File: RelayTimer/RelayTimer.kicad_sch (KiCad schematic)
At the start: 20 parts, among them J1 Jack-DC, J2 Relay_Con, Q1 2N3904, U1 ATtiny85-20P

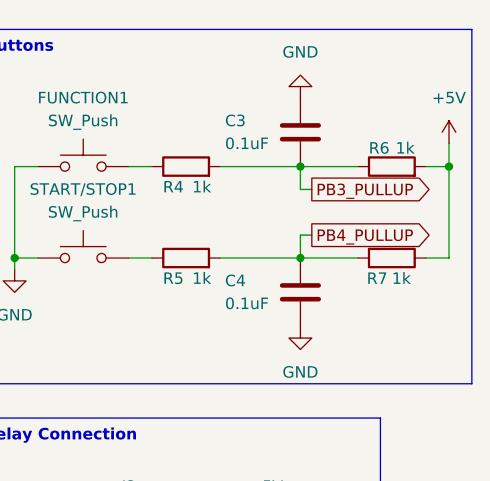
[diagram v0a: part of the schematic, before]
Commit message: minor update to KiCad project
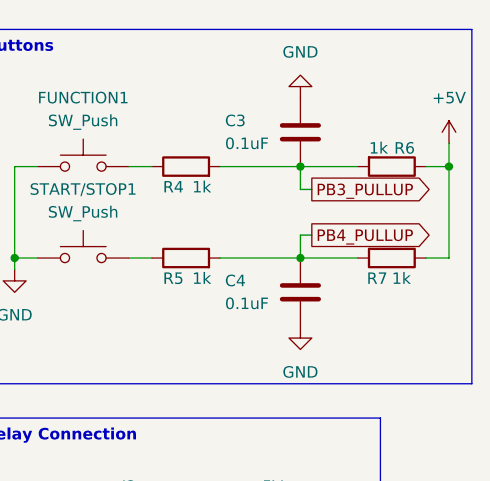
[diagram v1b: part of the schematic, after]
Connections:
- net +5V: now also R6.1; no longer R6.2
- net PB3_PULLUP: now also R6.2; no longer R6.1
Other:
- moved on the sheet: R6
